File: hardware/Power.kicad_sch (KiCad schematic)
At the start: 19 parts, among them U2 TPS61023DRL, U4 XC6206PxxxMR, U5 TOS2115ADRBT

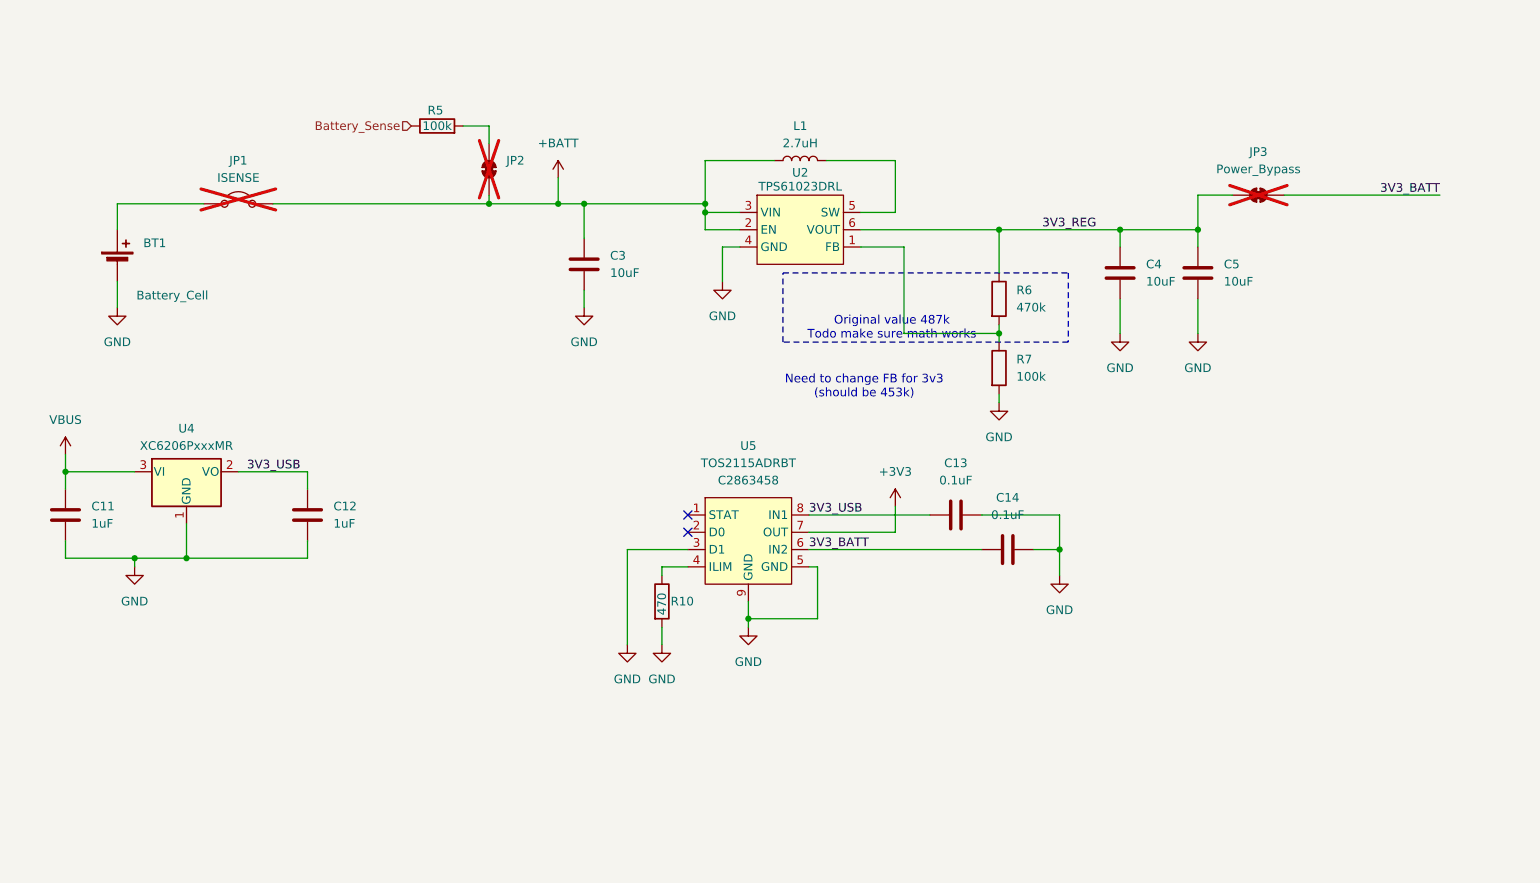
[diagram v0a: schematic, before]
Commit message: bom improvements
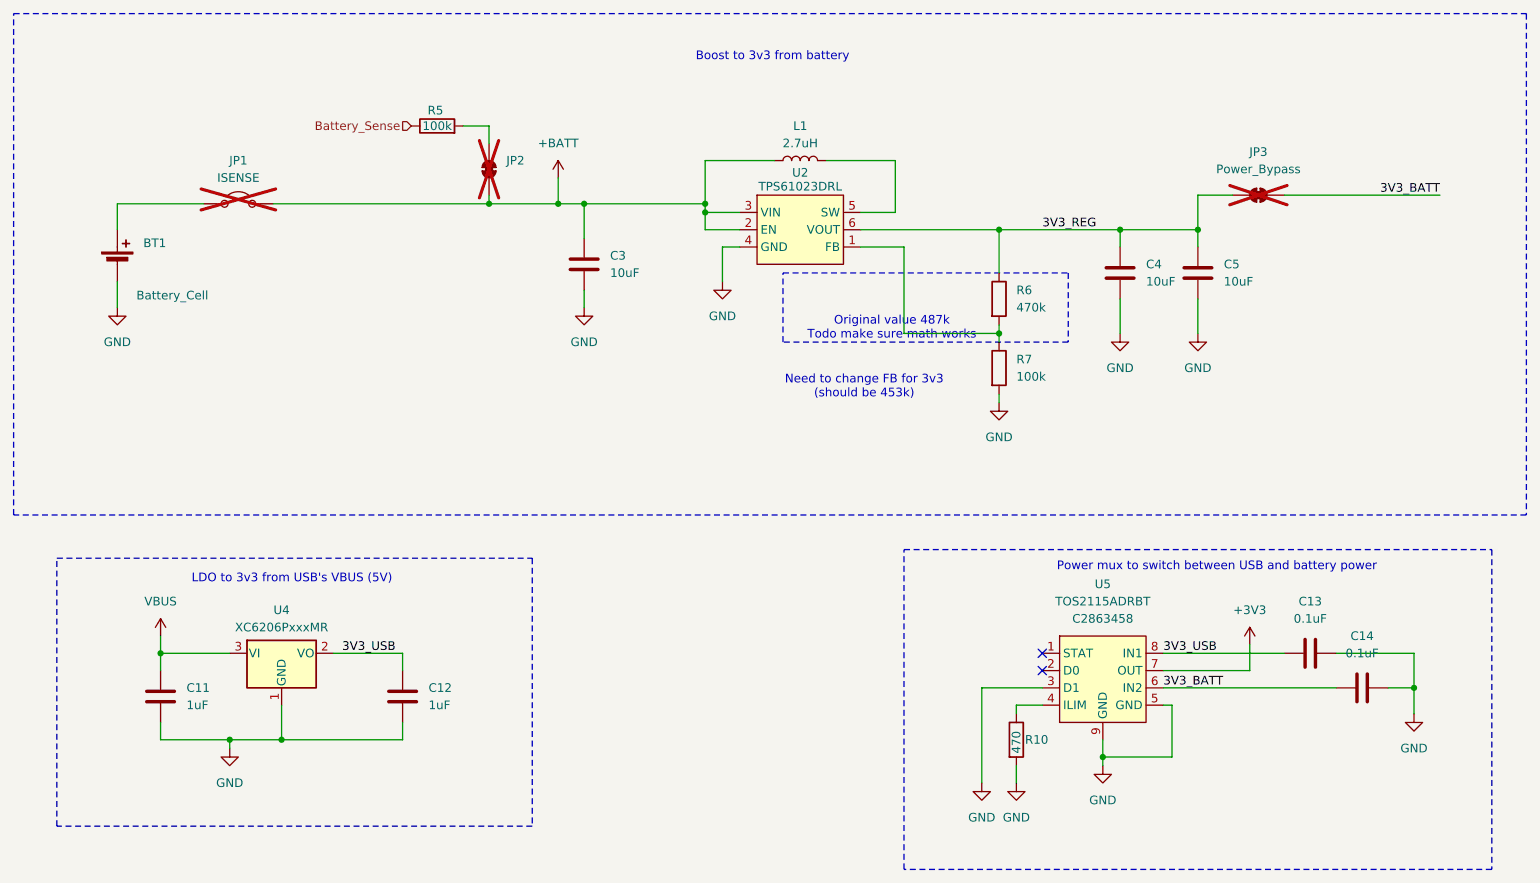
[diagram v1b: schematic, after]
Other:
- note added: "Boost to 3v3 from battery"
- note added: "LDO to 3v3 from USB's VBUS (5V)"
- note added: "Power mux to switch between USB and battery power"
- moved on the sheet: C11, C12, C13, C14, R10, U4, U5
